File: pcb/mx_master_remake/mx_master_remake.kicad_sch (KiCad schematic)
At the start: 4 parts, among them J1 SWD, J2 Battery, J3 Wheel Magnet, U1 BT840

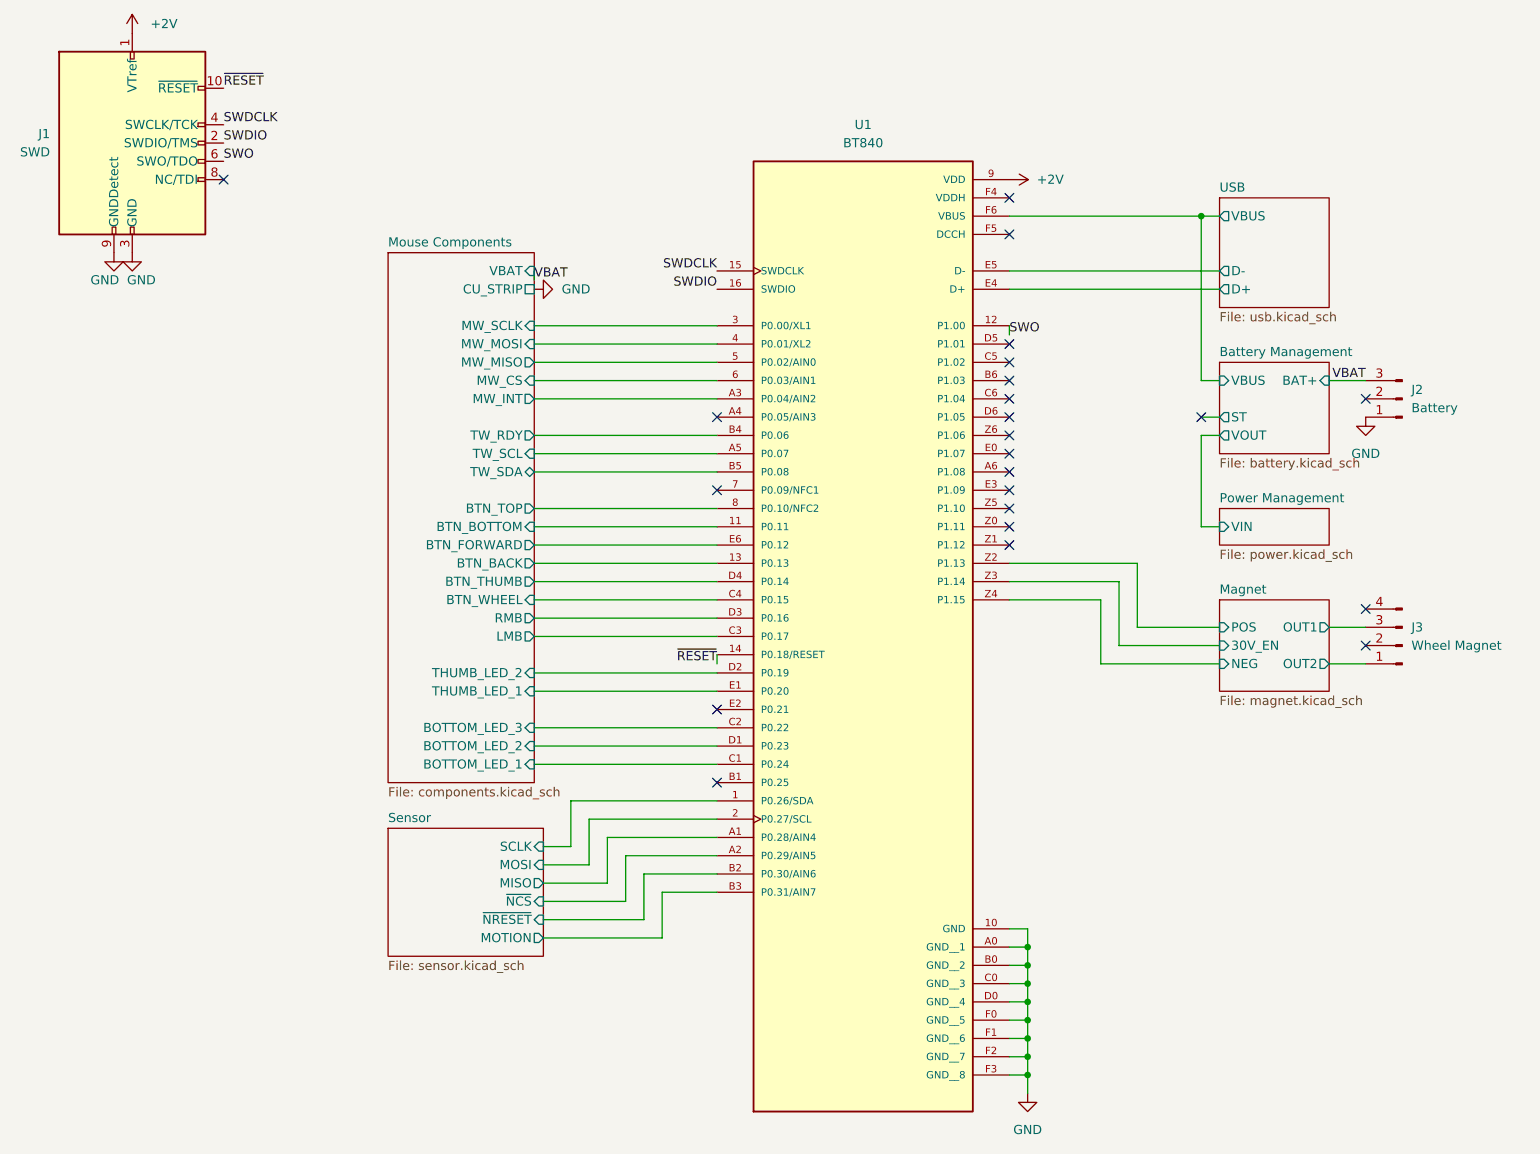
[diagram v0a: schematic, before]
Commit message: First
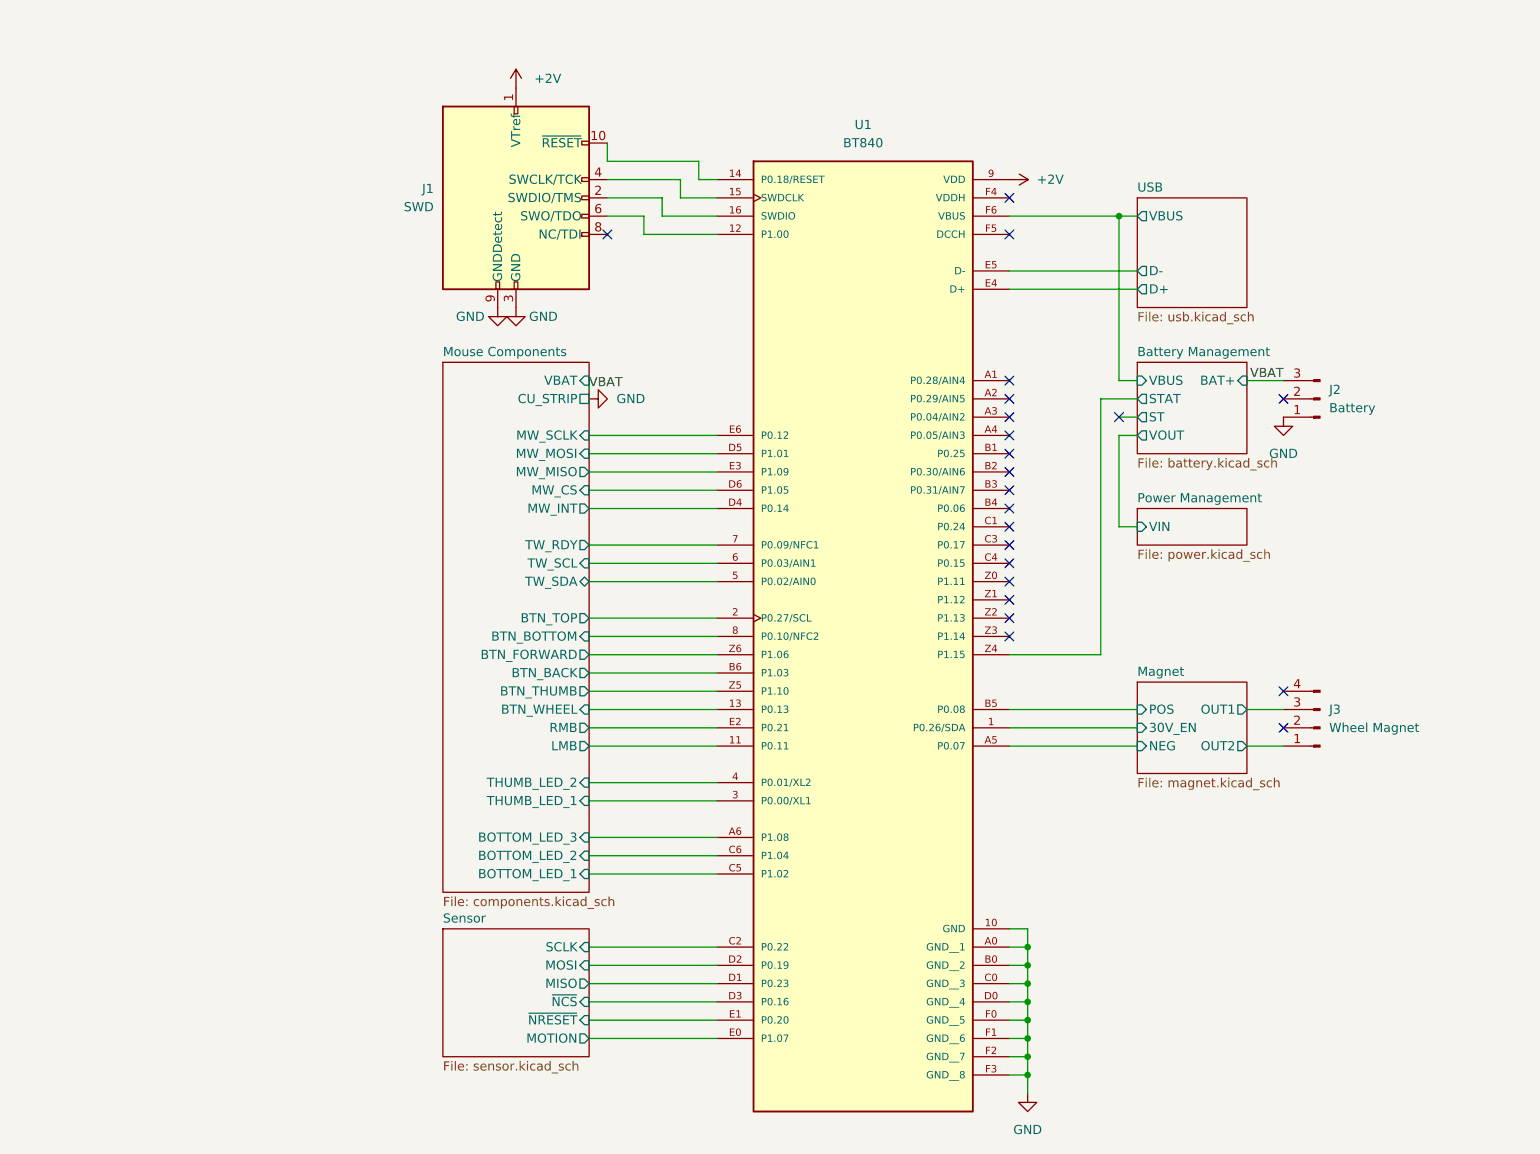
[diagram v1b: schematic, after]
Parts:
- removed U1: BT840, MCU:XCVR_BT840, symbol BT840:BT840
- added U1: BT840, MCU:XCVR_BT840, symbol BT840:BT840 Location Based Pins
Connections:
- net +2V0: now also U1.9 (VDD)
- net Battery Management/VBUS: now also U1.F6 (VBUS)
- net GND: now also U1.10 (GND), U1.A0 (GND__1), U1.B0 (GND__2), U1.C0 (GND__3), U1.D0 (GND__4), U1.F0 (GND__5), U1.F1 (GND__6), U1.F2 (GND__7), U1.F3 (GND__8)
- net Magnet/30V_EN: now also U1.1 (P0.26/SDA)
- net Magnet/NEG: now also U1.A5 (P0.07)
- net Magnet/POS: now also U1.B5 (P0.08)
- net Mouse Components/BOTTOM_LED_1: now also U1.C5 (P1.02)
- net Mouse Components/BOTTOM_LED_2: now also U1.C6 (P1.04)
- net Mouse Components/BOTTOM_LED_3: now also U1.A6 (P1.08)
- net Mouse Components/BTN_BACK: now also U1.B6 (P1.03)
- net Mouse Components/BTN_BOTTOM: now also U1.8 (P0.10/NFC2)
- net Mouse Components/BTN_FORWARD: now also U1.Z6 (P1.06)
- net Mouse Components/BTN_THUMB: now also U1.Z5 (P1.10)
- net Mouse Components/BTN_TOP: now also U1.2 (P0.27/SCL)
- net Mouse Components/BTN_WHEEL: now also U1.13 (P0.13)
- net Mouse Components/LMB: now also U1.11 (P0.11)
- net Mouse Components/MW_CS: now also U1.D6 (P1.05)
- net Mouse Components/MW_INT: now also U1.D4 (P0.14)
- net Mouse Components/MW_MISO: now also U1.E3 (P1.09)
- net Mouse Components/MW_MOSI: now also U1.D5 (P1.01)
- net Mouse Components/MW_SCLK: now also U1.E6 (P0.12)
- net Mouse Components/RMB: now also U1.E2 (P0.21)
- net Mouse Components/THUMB_LED_1: now also U1.3 (P0.00/XL1)
- net Mouse Components/THUMB_LED_2: now also U1.4 (P0.01/XL2)
- net Mouse Components/TW_RDY: now also U1.7 (P0.09/NFC1)
- net Mouse Components/TW_SCL: now also U1.6 (P0.03/AIN1)
- net Mouse Components/TW_SDA: now also U1.5 (P0.02/AIN0)
- net Sensor/MISO: now also U1.D1 (P0.23)
- net Sensor/MOSI: now also U1.D2 (P0.19)
- net Sensor/MOTION: now also U1.E0 (P1.07)
- net Sensor/SCLK: now also U1.C2 (P0.22)
- net Sensor/~{NCS}: now also U1.D3 (P0.16)
- net Sensor/~{NRESET}: now also U1.E1 (P0.20)
- net USB/D+: now also U1.E4 (D+)
- net USB/D-: now also U1.E5 (D-)
- net SWDCLK: no longer names the net of J1.4 (SWCLK/TCK)
- net SWDCLK: now also U1.15 (SWDCLK)
- net SWDIO: no longer names the net of J1.2 (SWDIO/TMS)
- net SWDIO: now also U1.16 (SWDIO)
- net SWO: no longer names the net of J1.6 (SWO/TDO)
- net SWO: now also U1.12 (P1.00)
- net ~{RESET}: no longer names the net of J1.10 (~{RESET})
- net ~{RESET}: now also U1.14 (P0.18/RESET)
- new net Battery Management/STAT: U1.Z4 (P1.15)
- no-connect marks 23 -> 22
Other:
- sheet Battery Management ports: added STAT; removed none
- moved on the sheet: J1, J2, J3
